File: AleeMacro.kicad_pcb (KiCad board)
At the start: 2 copper layers, 245.1 x 103.6 mm, 55 parts, among them U1 ProMicro

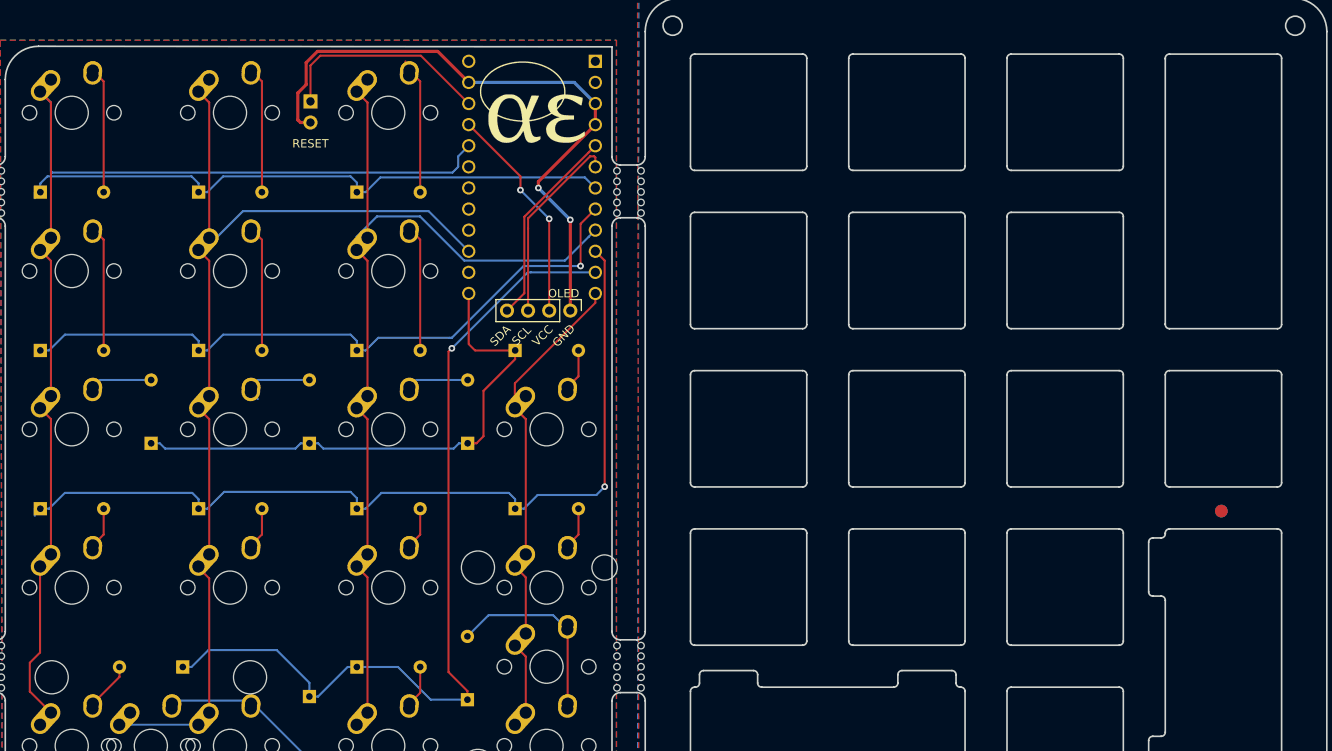
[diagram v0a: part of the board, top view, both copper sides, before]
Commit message: Routing Adjustments
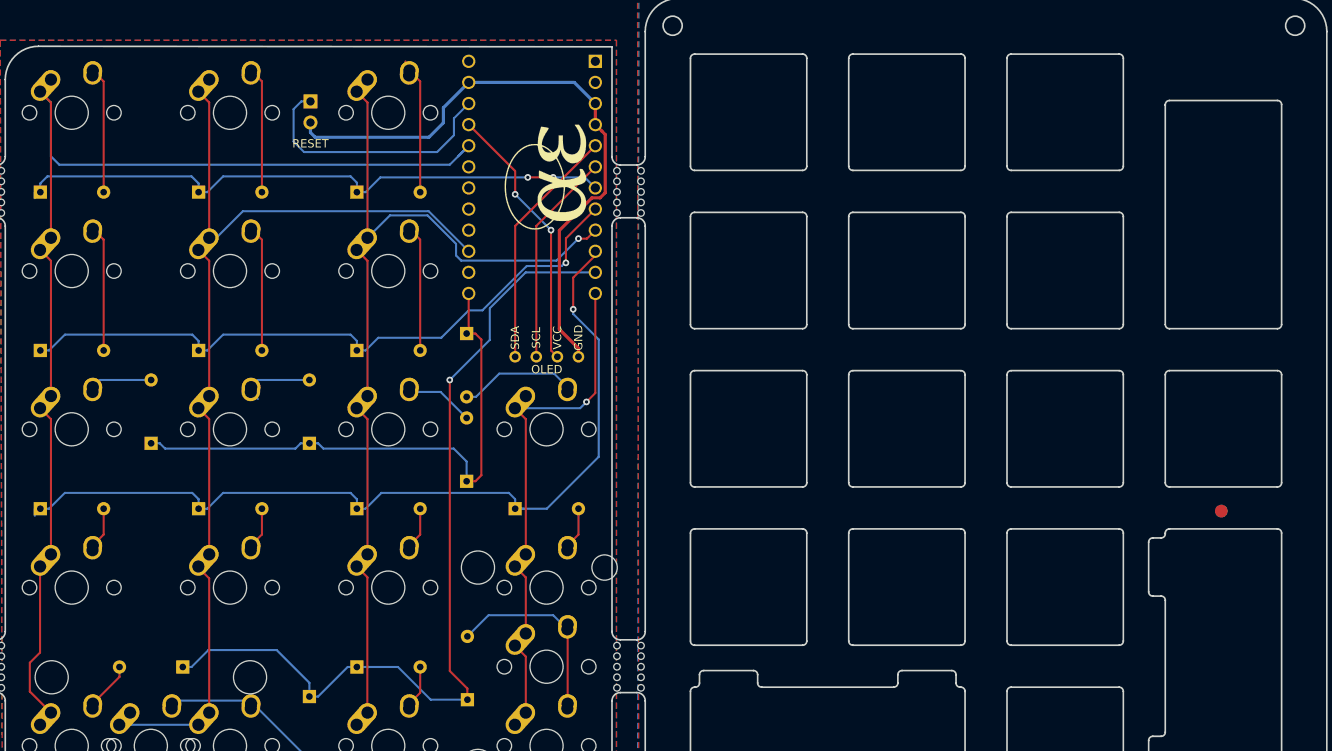
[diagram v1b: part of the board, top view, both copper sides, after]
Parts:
- OLED: footprint Connector_PinHeader_2.54mm:PinHeader_1x04_P2.54mm_Vertical -> kbd:OLED_v2
- moved G*** 9.07 mm to (177.0, 61.0), turned to 90 degrees
- moved OLED 7.39 mm to (177.0, 83.8), turned to 0 degrees
- moved D10 6.19 mm to (167.4, 79.8), turned to 270 degrees
- moved D9 4.57 mm to (167.4, 97.5)
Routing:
- net Net-(D12-Pad2): track 5.91 -> 15.5 mm
- net VCC: track 26.4 -> 32.4 mm
- net COL3: track 58.8 -> 64.6 mm, vias 0 -> 1
- net Net-(SW1-Pad1): track 26.2 -> 31.5 mm
- net SDA: track 24.2 -> 29.4 mm
- net SCL: track 23.5 -> 25.8 mm
- net ROW2: track 65.3 -> 67.2 mm
- net ROW1: track 81.3 -> 80.1 mm
- net GND: track 76.3 -> 75.4 mm, vias 2 -> 0
- net Net-(D11-Pad2): track 7.37 -> 8.23 mm
- net COL0: track 141.5 -> 140.7 mm
- net ROW3: track 105.6 -> 106.2 mm
- net COL2: track 117.7 -> 117.3 mm, vias 0 -> 1
- net ROW0: vias 0 -> 2
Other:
- outline, holes or cut-outs redrawn
- board text removed: "He touched the butt."
